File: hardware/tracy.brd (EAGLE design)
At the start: 50 x 38 mm, 80 parts, among them IC1 SIM900, J1 U.FL, J2 U.FL, Q4 si2305cd, T1 BC846, T2 BC846, U1 SPX5205 3v3, U2 3339, U3 TC1014 2V8, X1 MOLEX_2HORIZONTAL, X2 MOLEX_2HORIZONTAL, X3 MOLEX_6HORIZONTAL, X4 MOLEX_2HORIZONTAL, Y1 32768Hz CFPX-217 12.5pF

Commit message: manual update
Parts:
- C13: value 100n -> 100nF
- C14: value 22p -> 22pF
- U$1: value F55[0/1]X---PT48 -> MSP430F5510
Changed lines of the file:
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@@
 <element name="C6" library="rcl" package="C0805" value="100nF" x="38.2" y="11.1" rot="MR90"/>
 <element name="U$7" library="SparkFun" package="OSHW-LOGO-M" value="OSHW-LOGOM" x="9.35" y="5.92" rot="MR0"/>
-<element name="U$1" library="TI_MSP430_v16" package="PT48" value="F55[0/1]X---PT48" x="15.6" y="23.9" rot="MR90"/>
+<element name="U$1" library="TI_MSP430_v16" package="PT48" value="MSP430F5510" x="15.6" y="23.9" rot="MR90"/>
 <element name="C10" library="rcl" package="C0805" value="470nF" x="5.6" y="17.4" rot="MR270"/>
 <element name="Y1" library="Simplex-FreqCtrl" package="CRYSTAL-SMD-3.2X1.5" value="32768Hz CFPX-217 12.5pF" x="14.1" y="15.5" rot="MR180"/>
@@
 <element name="R15" library="rcl" package="R0805W" value="1k1" x="14.3" y="1.9" rot="R180"/>
 <element name="C12" library="rcl" package="C0805" value="4u7" x="34" y="21.55" rot="R90"/>
-<element name="C13" library="rcl" package="C0805" value="100n" x="34" y="25.7" rot="R90"/>
-<element name="C14" library="rcl" package="C0805" value="22p" x="42.7" y="9.65"/>
+<element name="C13" library="rcl" package="C0805" value="100nF" x="34" y="25.7" rot="R90"/>
+<element name="C14" library="rcl" package="C0805" value="22pF" x="42.7" y="9.65"/>
 <element name="T2" library="transistor" package="SOT23" value="BC846" x="3.1" y="9.3"/>
 <element name="R18" library="rcl" package="R0805W" value="47k" x="3.1" y="6.1" rot="R180"/>

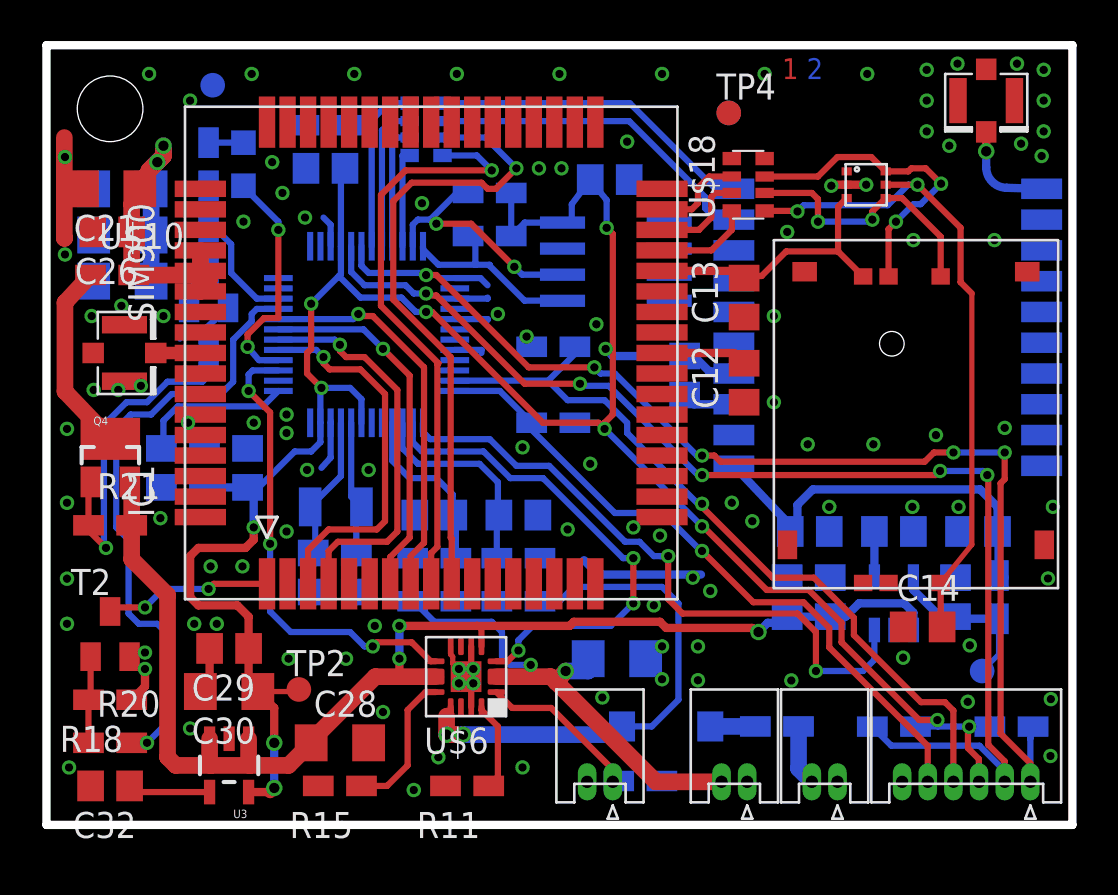
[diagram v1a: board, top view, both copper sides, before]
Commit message: latest
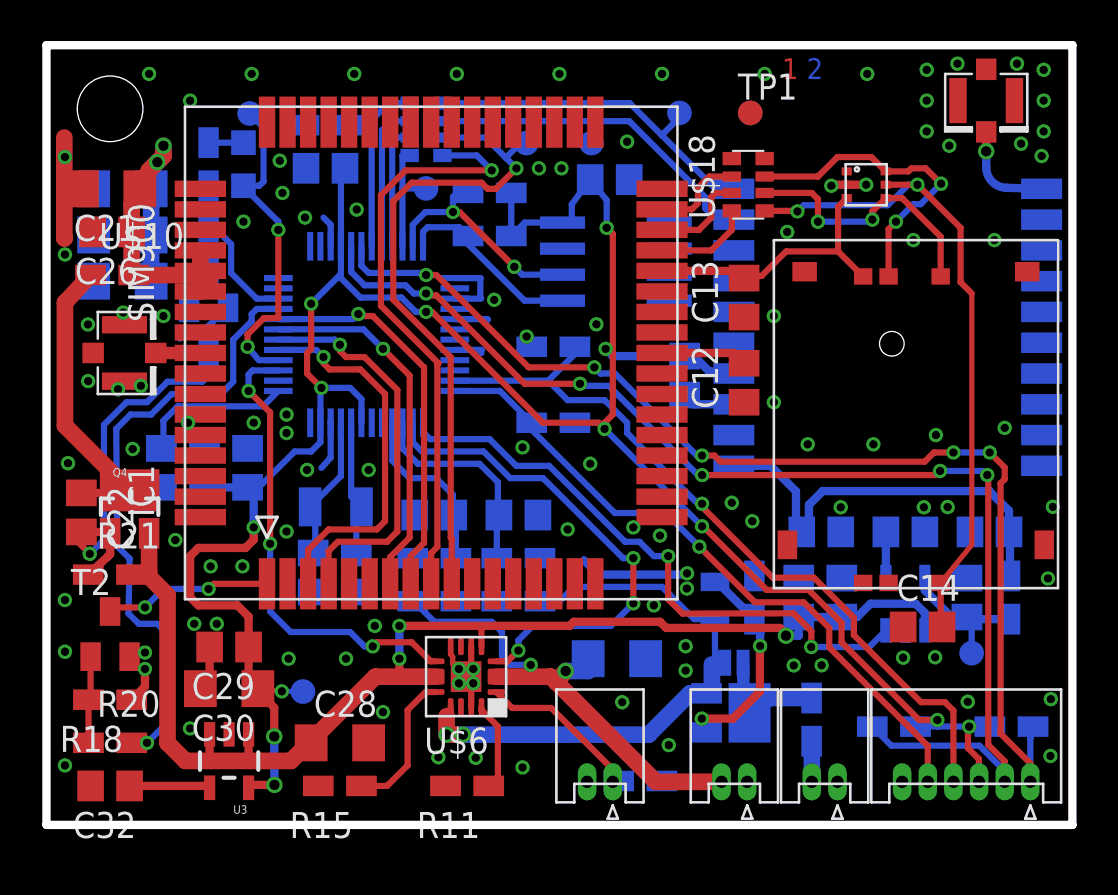
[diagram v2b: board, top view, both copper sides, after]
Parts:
- added C22: 100nF, rcl:C0805
- added JP1: no_prot, SparkFun-Passives:SJ_2S-NO
- added Q1: si2305cd, Simplex-DiscreteSemi:SOT23-3_POWER
- added R9: 4k7, rcl:R0805W
- added TP1, TP101, TP102, TP103: TPTP12R, testpad:TP12R
- D1: value 15MQ040N -> bzm55c5v6; device SparkFun-DiscreteSemi:SMA-DIODE -> diode:MICROMELF-W
- R21: value 10k -> 100k
- moved TP2 33.7 mm to (30.9, 34.7), flipped to the bottom
- moved TP3 32.0 mm to (26.6, 33.2)
- moved TP6 23.4 mm to (9.90, 34.7)
- moved TP5 11.6 mm to (18.5, 31.0)
- moved TP4 9.97 mm to (23.4, 33.2), flipped to the bottom
- moved D1 6.54 mm to (32.6, 10.9), turned to 90 degrees
- moved Q4 2.68 mm to (4.04, 15.6)
- moved R21 2.40 mm to (3.09, 12.2)
- moved U$9 1.72 mm to (37.3, 5.13), turned to 90 degrees
- moved U$7 1.11 mm to (8.62, 6.75)
- moved C4 0.56 mm to (41.9, 14.3)
- moved C5 0.56 mm to (46.0, 14.3)
- moved U1 0.56 mm to (41.9, 10.8)
- moved C1 0.56 mm to (44.9, 11.1)
- moved U$5 0.56 mm to (47.0, 11.1)
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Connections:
- net CH renamed CHG
- removed net N$20: D1.A, U$9.2
- new net N$11: D1.A, Q1.1, R9.1
- new net N$5: JP1.1, Q1.3, U$9.2
- net +3V3: now also TP103.TP; no longer TP3.TP
- net 2V8: now also TP102.TP; no longer TP2.TP
- net 5V_IN: now also JP1.2, Q1.2
- net GND: now also R9.2, TP1.TP, TP101.TP; no longer TP4.TP, TP5.TP, TP6.TP
- net GPRS_RX: now also TP4.TP
- net GPS_RX: now also TP2.TP
- net GPS_TX: now also TP3.TP
- net N$10: now also TP5.TP
- net N$48: now also C22.2
- net N$49: now also C22.1
- net STATUS: now also TP6.TP
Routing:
- net N$11: track 0.00 -> 10.9 mm, vias 0 -> 2
- net N$5: track 0.00 -> 5.83 mm
- net N$49: track 9.36 -> 14.7 mm
- net STATUS: track 11.4 -> 16.0 mm
- net 5V_IN: track 26.1 -> 29.5 mm
- net N$48: track 16.8 -> 19.4 mm
- net N$20: track 2.20 -> 0.00 mm
- net 3V3_EN: track 31.7 -> 29.8 mm
- net GPS_VCC: track 20.3 -> 21.9 mm
- net GPS_RX: track 15.9 -> 17.4 mm
- net GPRS_RX: track 31.0 -> 32.3 mm
- net N$10: track 4.77 -> 5.92 mm
- net GPS_TX: track 16.6 -> 17.6 mm
- net +3V3: track 8.26 -> 7.24 mm
- net 5V: track 2.97 -> 1.98 mm
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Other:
- board text added: "Petre Rodan 201411 rev2.1"
- board text added: "tp1"
- board text added: "tp2"
- board text added: "tp3"
- board text added: "tp4"
- board text added: "tp5"
- board text added: "tp6"
- board text removed: "Petre Rodan 201408 rev2"
